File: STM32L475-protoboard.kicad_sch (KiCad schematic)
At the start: 75 parts, among them J1 USB_HEADER, J10 BOOT_MODE, J11 PAD_PB4, J12 PAD_PB5, J13 PAD_PC4, J14 PAD_PC5, J15 Micro_SD_Card, J16 Conn_02x20_Odd_Even, J2 USB_B_Micro, J3 DCin, J4 STLINK, J5 W5500_ETHERNET, J6 STLINK2, J7 PAD_PA9_USART1_TX, J8 PAD_PA10_USART1_RX, J9 GNDPAD, SW1 RESET, U1 SRV05-4, U2 AMS1117-3.3, U3 STM32L475RCTx, Y1 16 MHz, Y2 32.768k

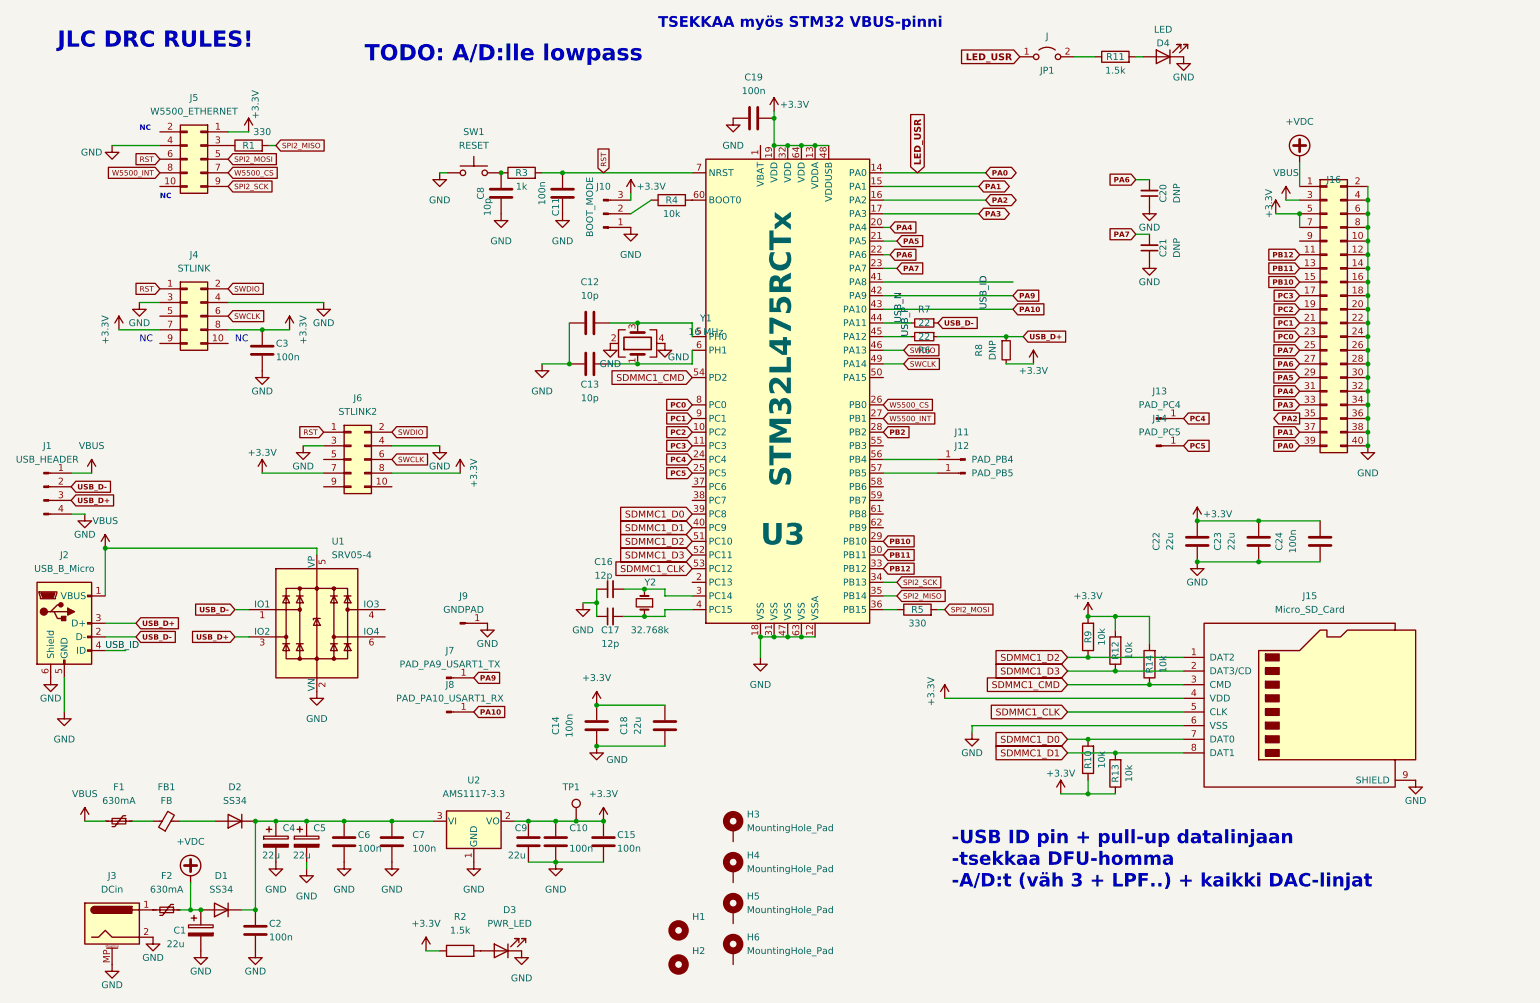
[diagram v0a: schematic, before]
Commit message: microsd + misc
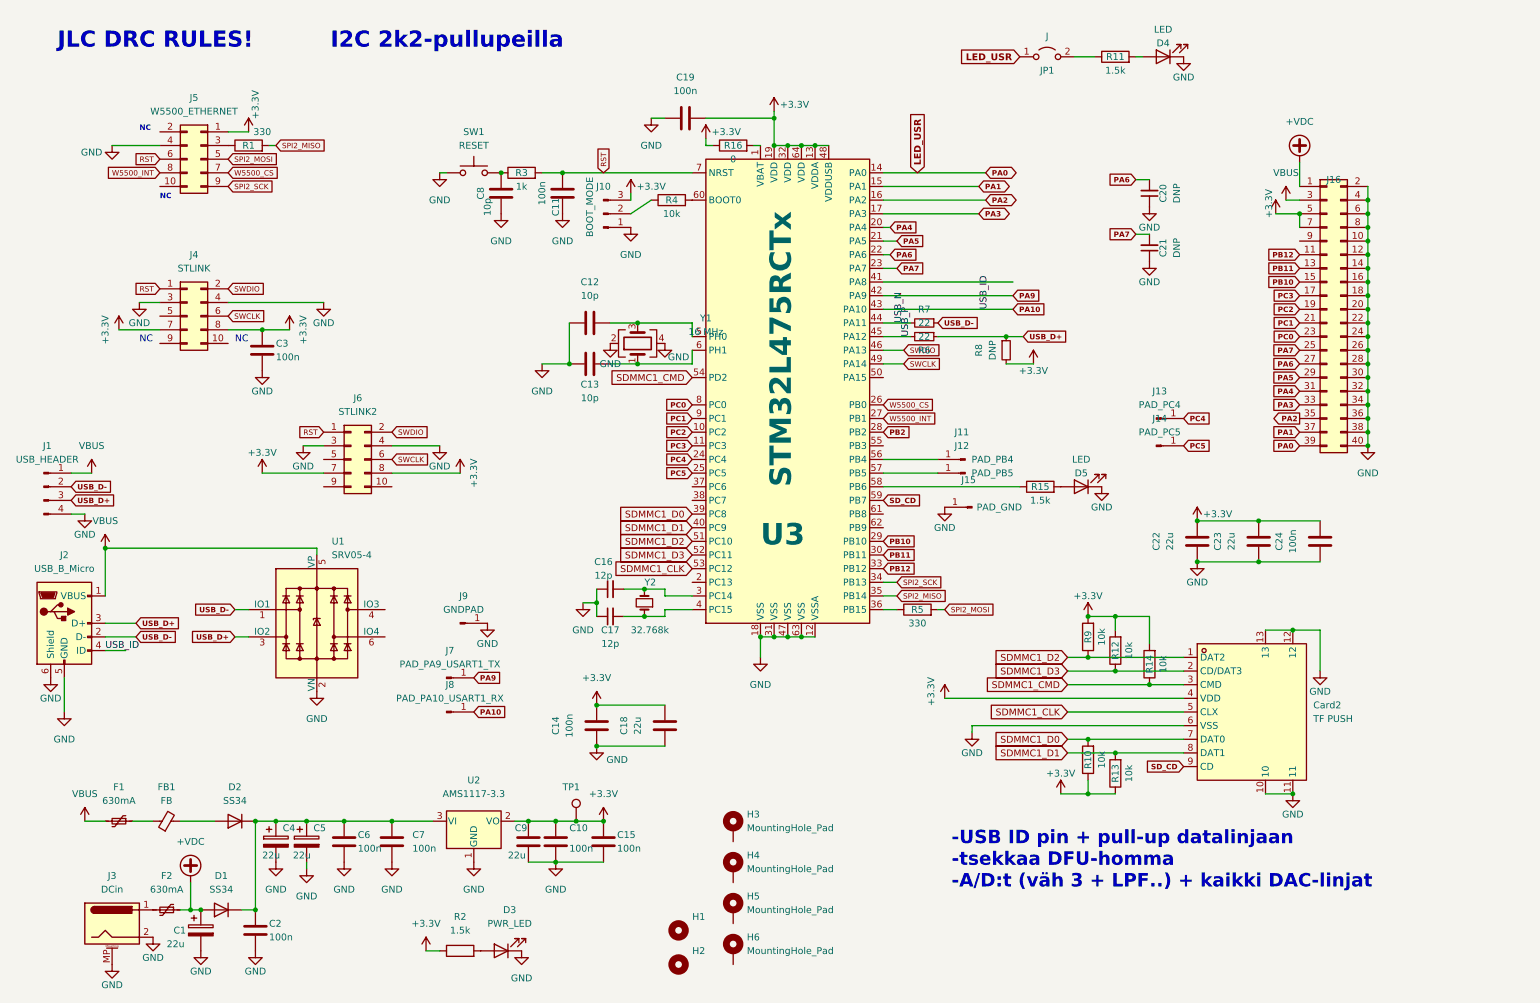
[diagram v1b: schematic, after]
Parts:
- removed J15: Micro_SD_Card, Connector_Card:microSD_HC_Wuerth_693072010801, symbol Connector:Micro_SD_Card
- added Card2: TF PUSH, STM32L475-protoboard:TF-SMD_TF-PUSH, symbol easyeda2kicad:TFPUSH
- added D5: LED, LED_SMD:LED_0805_2012Metric, symbol Device:LED
- added J15: PAD_GND, Connector_Wire:SolderWirePad_1x01_SMD_1x2mm, symbol Connector:Conn_01x01_Male
- added R15: 1.5k, Resistor_SMD:R_0603_1608Metric_Pad0.98x0.95mm_HandSolder, symbol Device:R
- added R16: 0, Resistor_SMD:R_0603_1608Metric_Pad0.98x0.95mm_HandSolder, symbol Device:R
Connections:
- net +3V3: now also Card2.4 (VDD), R16.1
- net GND: now also Card2.10, Card2.11, Card2.12, Card2.13, Card2.6 (VSS), D5.1 (K), J15.1 (Pin_1)
- net SDMMC1_CLK: now also Card2.5 (CLX)
- net SDMMC1_CMD: now also Card2.3 (CMD)
- net SDMMC1_D0: now also Card2.7 (DAT0)
- net SDMMC1_D1: now also Card2.8 (DAT1)
- net SDMMC1_D2: now also Card2.1 (DAT2)
- net SDMMC1_D3: now also Card2.2 (CD/DAT3)
- net at U3.1 (VBAT): now also R16.2
- net at U3.58 (PB6): now also R15.1
- net SD_CD: now reaches U3.59 (PB7)
- net SD_CD: now also Card2.9 (CD)
- new net: D5.2 (A), R15.2
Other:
- note added: "I2C 2k2-pullupeilla"
- note removed: "TODO: A/D:lle lowpass"
- note removed: "TSEKKAA myös STM32 VBUS-pinni"
- moved on the sheet: C19
